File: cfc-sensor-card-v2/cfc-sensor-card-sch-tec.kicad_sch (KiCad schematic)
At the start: 32 parts, among them U12 AD5593RBCPZ-RL7, U15 MP2410A, U16 DRV8212DSGR, U17 INA186A1IDCKR

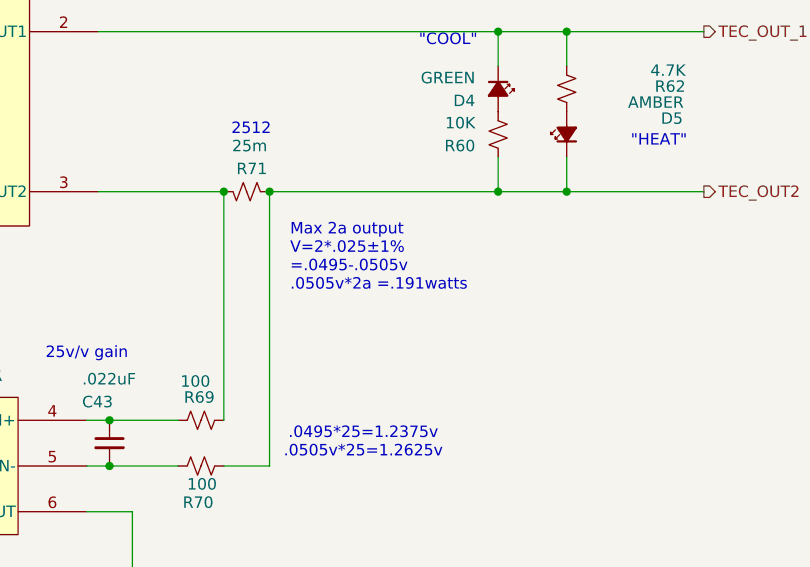
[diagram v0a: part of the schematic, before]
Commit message: Update
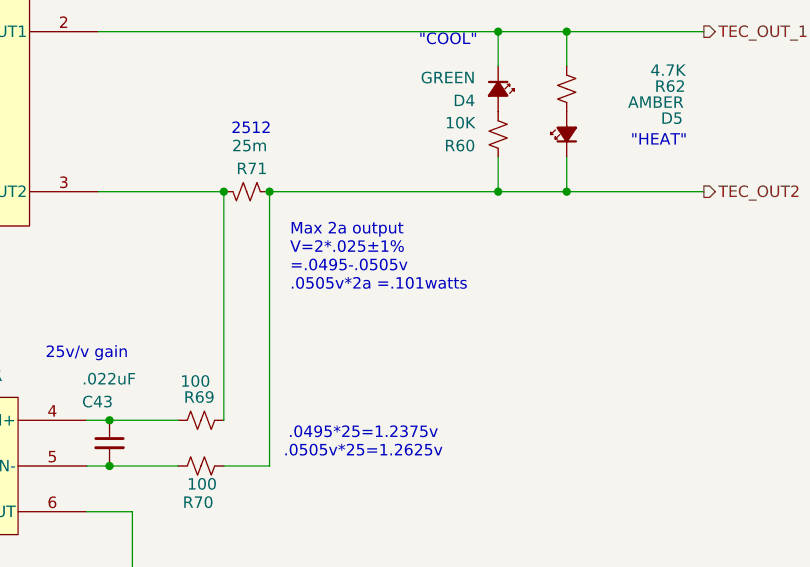
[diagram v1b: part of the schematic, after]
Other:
- note added: "Max 2a output V=2*.025±1% =.0495-.0505v .0505v*2a =.101watts"
- note removed: "Max 2a output V=2*.025±1% =.0495-.0505v .0505v*2a =.191watts"
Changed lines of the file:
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@@
 		)
 	)
-	(text "Max 2a output\nV=2*.025±1%\n=.0495-.0505v\n.0505v*2a =.191watts "
+	(text "Max 2a output\nV=2*.025±1%\n=.0495-.0505v\n.0505v*2a =.101watts "
 		(exclude_from_sim no)
 		(at 332.486 186.436 0)

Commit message: Revert "Update"
This reverts commit deafafed1fe993a788287949c9b0e14f8f1b09d1.
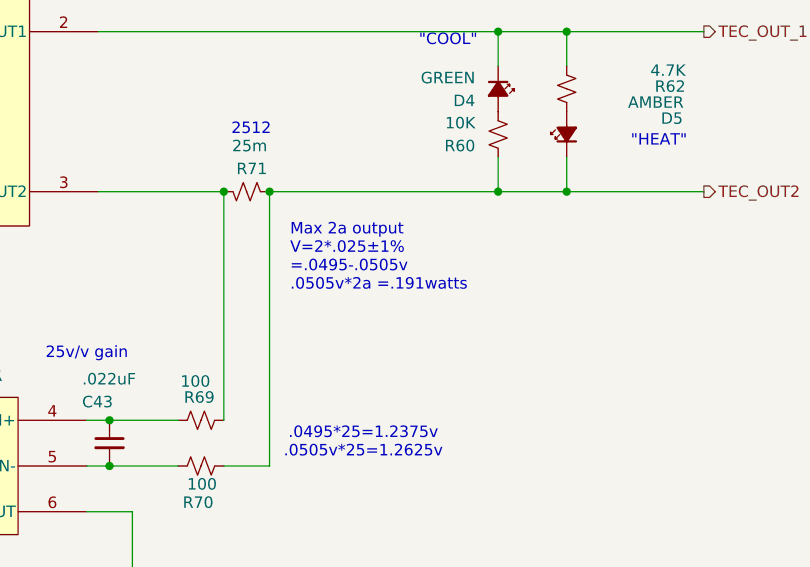
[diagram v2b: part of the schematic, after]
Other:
- note added: "Max 2a output V=2*.025±1% =.0495-.0505v .0505v*2a =.191watts"
- note removed: "Max 2a output V=2*.025±1% =.0495-.0505v .0505v*2a =.101watts"
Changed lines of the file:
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@@
 		)
 	)
-	(text "Max 2a output\nV=2*.025±1%\n=.0495-.0505v\n.0505v*2a =.101watts "
+	(text "Max 2a output\nV=2*.025±1%\n=.0495-.0505v\n.0505v*2a =.191watts "
 		(exclude_from_sim no)
 		(at 332.486 186.436 0)
